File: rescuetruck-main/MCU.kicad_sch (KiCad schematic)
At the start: 24 parts, among them IC1 W25Q16JVUXIQ, SW1 Reset, U3 RP2040, Y1 JGHC S3212000181080

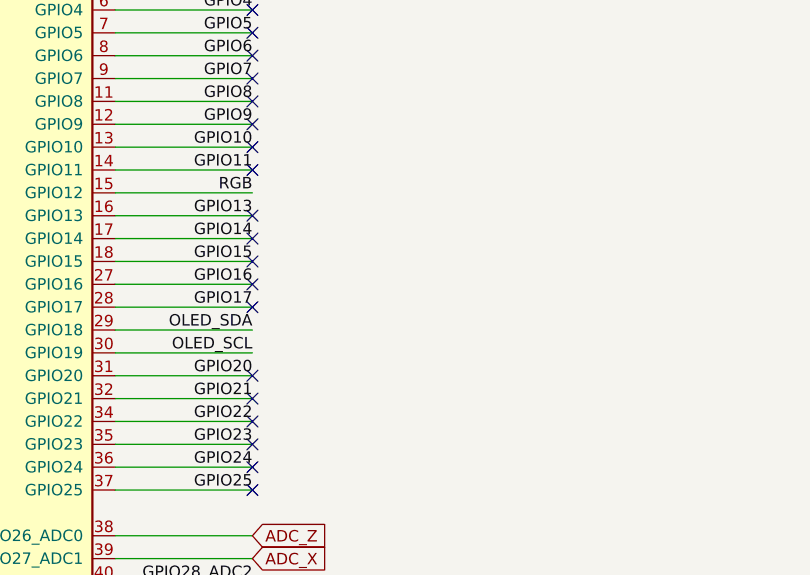
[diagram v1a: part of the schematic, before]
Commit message: vootvan progress
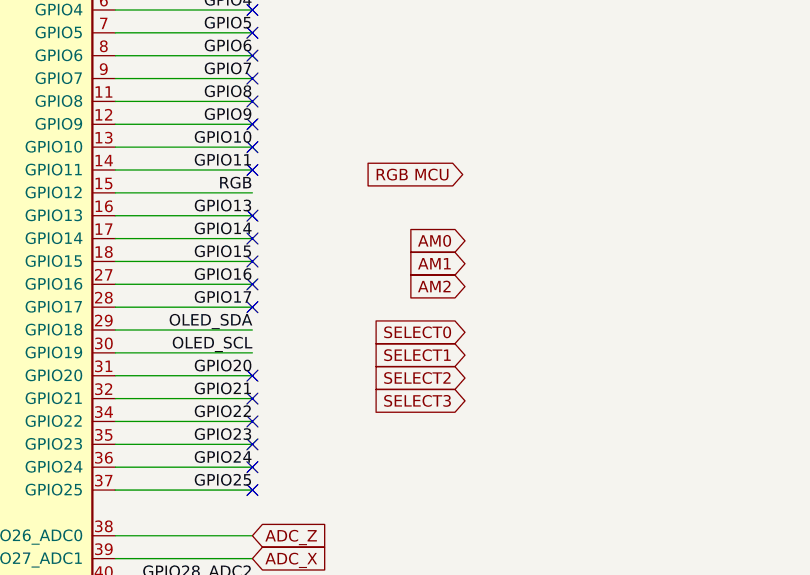
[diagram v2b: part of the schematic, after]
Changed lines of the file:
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@@
     (effects (font (size 1.27 1.27)) (justify right bottom))
+  )
+  (global_label "SELECT1" (shape input) (at 142.24 124.46 180) (fields_autoplaced)
+    (effects (font (size 1.27 1.27)) (justify right))
+    (property "Intersheetrefs" "${INTERSHEET_REFS}" (at 132.0057 124.46 0)
+      (effects (font (size 1.27 1.27)) (justify right) hide)
+    )
+  )
+  (global_label "SELECT3" (shape input) (at 142.24 129.54 180) (fields_autoplaced)
+    (effects (font (size 1.27 1.27)) (justify right))
+    (property "Intersheetrefs" "${INTERSHEET_REFS}" (at 132.0057 129.54 0)
+      (effects (font (size 1.27 1.27)) (justify right) hide)
+    )
+  )
+  (global_label "SELECT0" (shape input) (at 142.24 121.92 180) (fields_autoplaced)
+    (effects (font (size 1.27 1.27)) (justify right))
+    (property "Intersheetrefs" "${INTERSHEET_REFS}" (at 132.0057 121.92 0)
+      (effects (font (size 1.27 1.27)) (justify right) hide)
+    )
+  )
+  (global_label "SELECT2" (shape input) (at 142.24 127 180) (fields_autoplaced)
+    (effects (font (size 1.27 1.27)) (justify right))
+    (property "Intersheetrefs" "${INTERSHEET_REFS}" (at 132.0057 127 0)
+      (effects (font (size 1.27 1.27)) (justify right) hide)
+    )
+  )
+  (global_label "AM0" (shape input) (at 142.24 111.76 180) (fields_autoplaced)
+    (effects (font (size 1.27 1.27)) (justify right))
+    (property "Intersheetrefs" "${INTERSHEET_REFS}" (at 136.2389 111.76 0)
+      (effects (font (size 1.27 1.27)) (justify right) hide)
+    )
+  )
+  (global_label "RGB MCU" (shape input) (at 141.986 104.394 180) (fields_autoplaced)
+    (effects (font (size 1.27 1.27)) (justify right))
+    (property "Intersheetrefs" "${INTERSHEET_REFS}" (at 131.1105 104.394 0)
+      (effects (font (size 1.27 1.27)) (justify right) hide)
+    )
   )
   (global_label "USB_D+" (shape input) (at 125.222 60.706 0) (fields_autoplaced)
@@
     )
   )
+  (global_label "AM2" (shape input) (at 142.24 116.84 180) (fields_autoplaced)
+    (effects (font (size 1.27 1.27)) (justify right))
+    (property "Intersheetrefs" "${INTERSHEET_REFS}" (at 136.2389 116.84 0)
+      (effects (font (size 1.27 1.27)) (justify right) hide)
+    )
+  )
   (global_label "USB_D-" (shape input) (at 125.222 68.326 0) (fields_autoplaced)
     (effects (font (size 1.27 1.27)) (justify left))
@@
     )
   )
+  (global_label "AM1" (shape input) (at 142.24 114.3 180) (fields_autoplaced)
+    (effects (font (size 1.27 1.27)) (justify right))
+    (property "Intersheetrefs" "${INTERSHEET_REFS}" (at 136.2389 114.3 0)
+      (effects (font (size 1.27 1.27)) (justify right) hide)
+    )
+  )
